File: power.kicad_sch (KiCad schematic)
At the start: 29 parts, among them J2 USB_C_Receptacle, Q1 Q_NMOS_GSD, Q2 Q_NMOS_GSD, Q3 DMG2301L, U3 MCP73831-2-OT, U4 MAX17048, U8 LD39150DT33

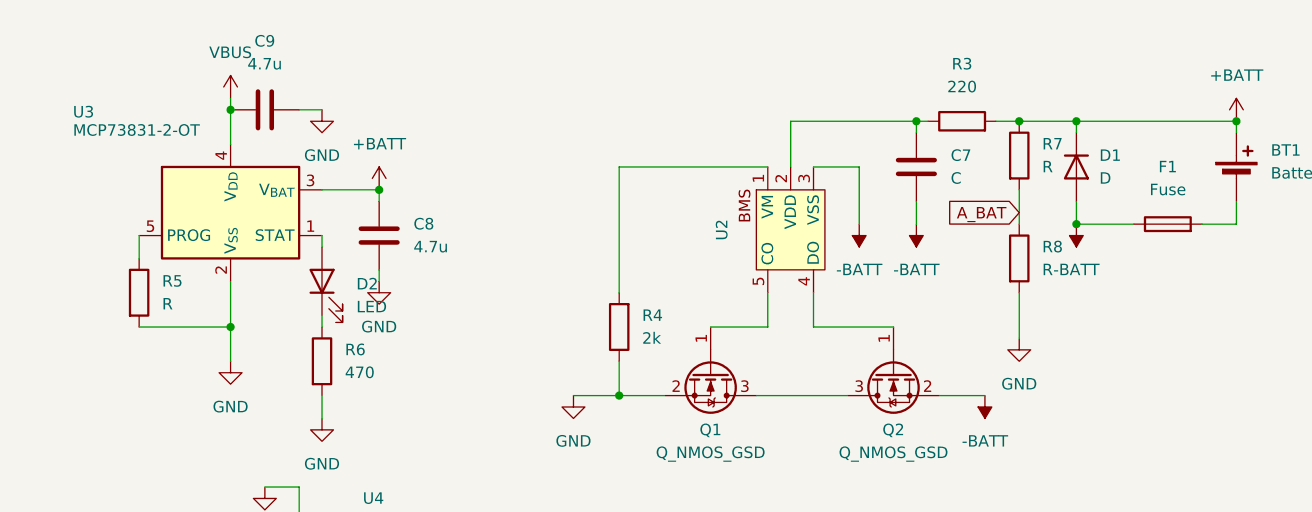
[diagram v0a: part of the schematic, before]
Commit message: finished schematic
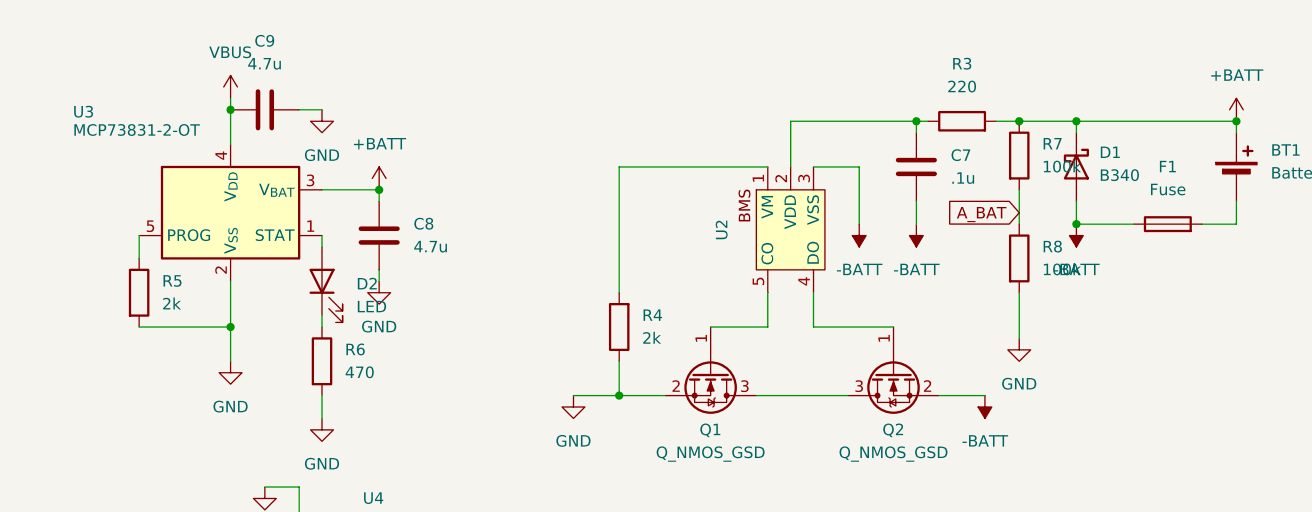
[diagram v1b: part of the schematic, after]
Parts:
- removed D1: D, symbol Device:D
- added D1: B340, Diode_SMD:D_SMC, symbol Diode:B340
- C10: footprint (none) -> Capacitor_SMD:C_0603_1608Metric; LCSC PN (none) -> C14663
- C19, C20: footprint (none) -> Capacitor_SMD:C_0603_1608Metric; LCSC PN (none) -> C15849
- C7: value C -> .1u; footprint (none) -> Capacitor_SMD:C_0603_1608Metric; LCSC PN (none) -> C14663
- C8, C9: footprint (none) -> Capacitor_SMD:C_0603_1608Metric; LCSC PN (none) -> C19666
- D2: footprint (none) -> LED_SMD:LED_0805_2012Metric; LCSC PN (none) -> C965817
- F1: LCSC PN C2982275 -> C135349; Part Number Shenzhen JDT Fuse ASMD1210-150-16V -> Shenzhen JDT Fuse ASMD1210-075
- R1, R2: footprint (none) -> Resistor_SMD:R_0603_1608Metric; LCSC PN (none) -> C122969
- R3: footprint (none) -> Resistor_SMD:R_0603_1608Metric; LCSC PN (none) -> C107696
- R4: footprint (none) -> Resistor_SMD:R_0603_1608Metric; LCSC PN (none) -> C105576
- R5: value R -> 2k; footprint (none) -> Resistor_SMD:R_0603_1608Metric; LCSC PN (none) -> C105576
- R6: footprint (none) -> Resistor_SMD:R_0603_1608Metric; LCSC PN (none) -> C114669
- R7, R8: value R -> 100k; footprint (none) -> Resistor_SMD:R_0603_1608Metric; LCSC PN (none) -> C14675
- R9: footprint (none) -> Resistor_SMD:R_0603_1608Metric; LCSC PN (none) -> C14675
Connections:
- net +BATT: now also D1.1 (K)
- net -BATT: now also D1.2 (A)
